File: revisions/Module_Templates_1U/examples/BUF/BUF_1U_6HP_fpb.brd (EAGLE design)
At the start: 28.4 x 28.4 mm, 11 parts, among them J2 ERA-NOSILK

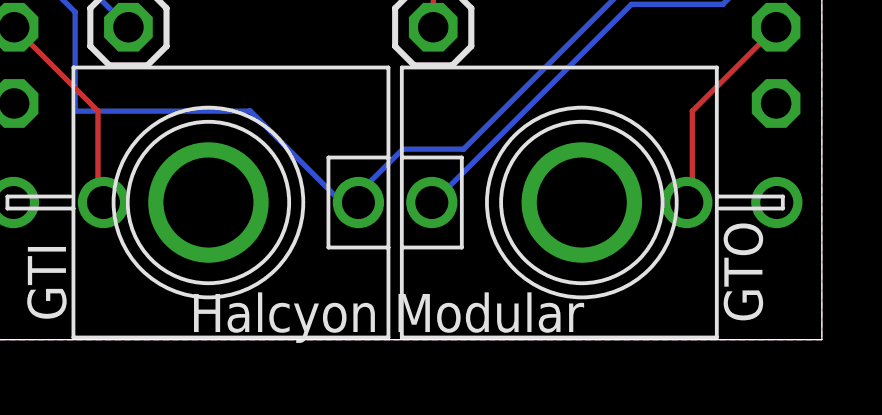
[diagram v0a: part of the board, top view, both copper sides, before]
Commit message: Update Backplane Reference
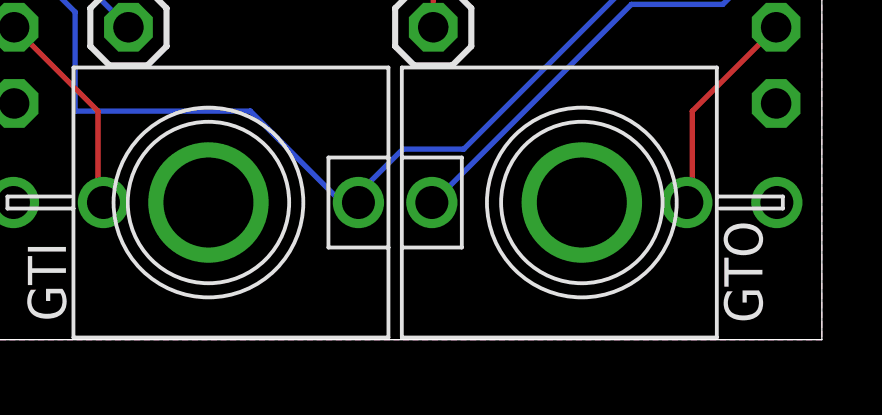
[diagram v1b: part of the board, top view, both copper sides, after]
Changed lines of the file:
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@@
 <setting verticaltext="up"/>
 </settings>
-<grid distance="10" unitdist="mil" unit="mil" style="lines" multiple="10" display="yes" altdistance="0.025" altunitdist="inch" altunit="inch"/>
+<grid distance="10" unitdist="mil" unit="mm" style="lines" multiple="10" display="yes" altdistance="0.025" altunitdist="inch" altunit="inch"/>
 <layers>
 <layer number="1" name="Top" color="4" fill="1" visible="no" active="yes"/>
@@
 <layer number="220" name="220bmp" color="21" fill="1" visible="no" active="no"/>
 <layer number="221" name="221bmp" color="22" fill="1" visible="no" active="no"/>
-<layer number="222" name="222bmp" color="23" fill="1" visible="no" active="no"/>
 <layer number="223" name="223bmp" color="24" fill="1" visible="no" active="no"/>
 <layer number="224" name="224bmp" color="25" fill="1" visible="no" active="no"/>
@@
 <circle x="5.08" y="40.1828" radius="1.905" width="0.4064" layer="51"/>
 <circle x="5.08" y="2.9972" radius="1.9235375" width="0.4064" layer="51"/>
-<text x="8.382" y="7.62" size="1.27" layer="21" font="vector" ratio="20">Halcyon Modular</text>
 <text x="23.876" y="8.89" size="1.27" layer="22" font="vector" ratio="20" rot="R180">Halcyon Modular</text>
 </plain>
